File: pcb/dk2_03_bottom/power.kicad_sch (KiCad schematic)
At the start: 11 parts, among them J3 Eurorack_Power, U2 AP7333-33SAG, U8 XL1509-5.0

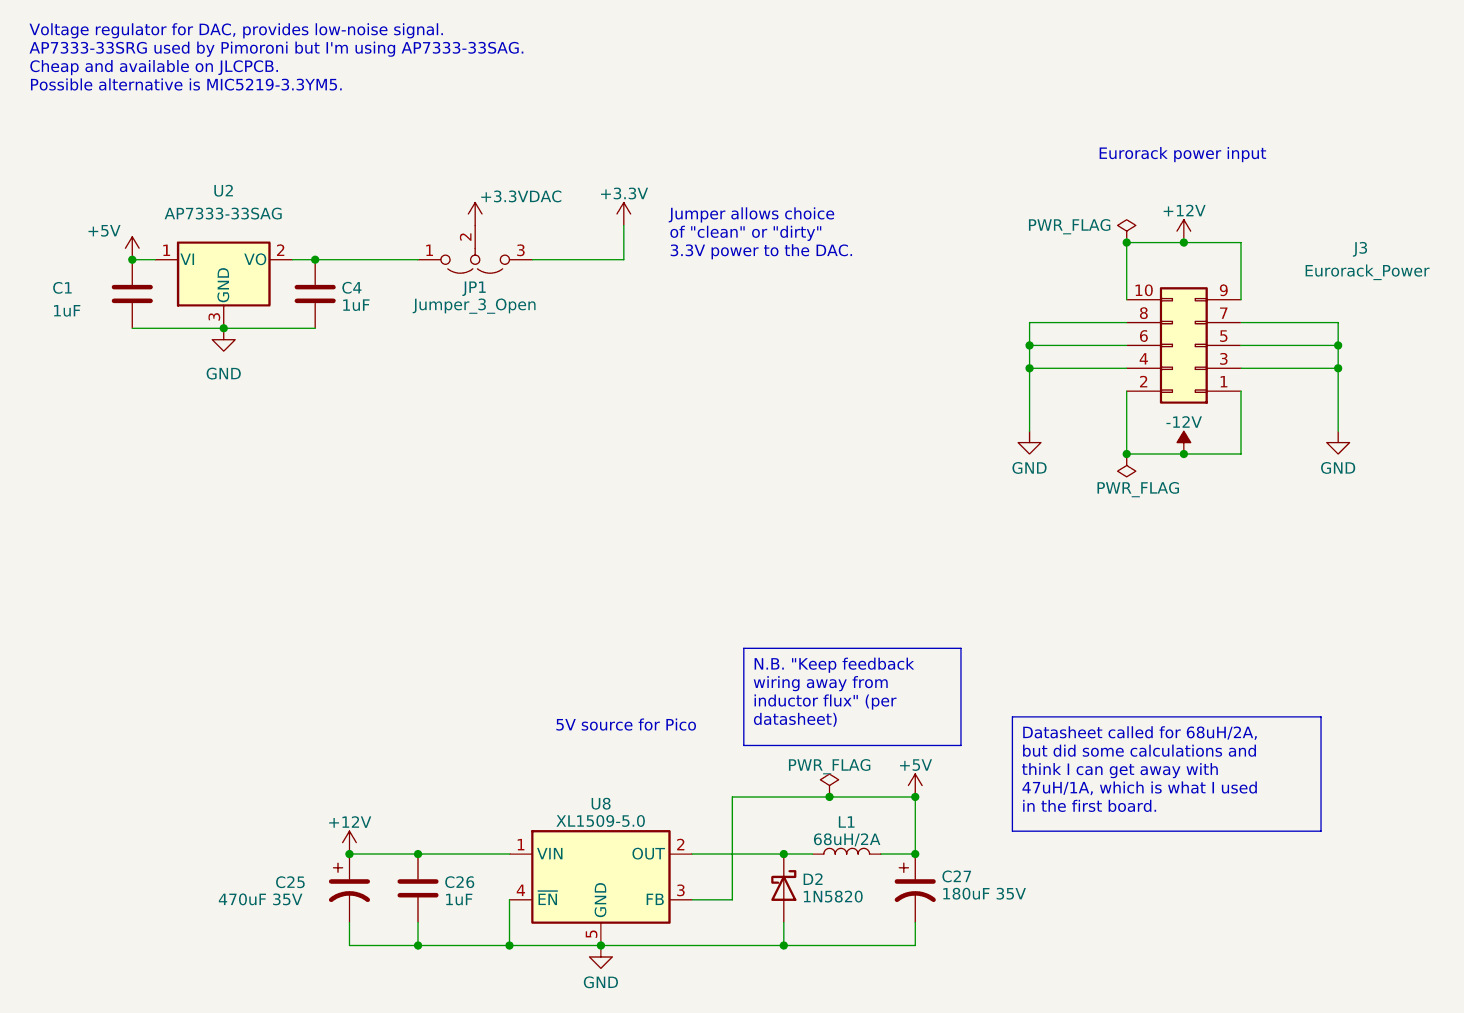
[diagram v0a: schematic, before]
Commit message: a commit before i mess up all the buttons
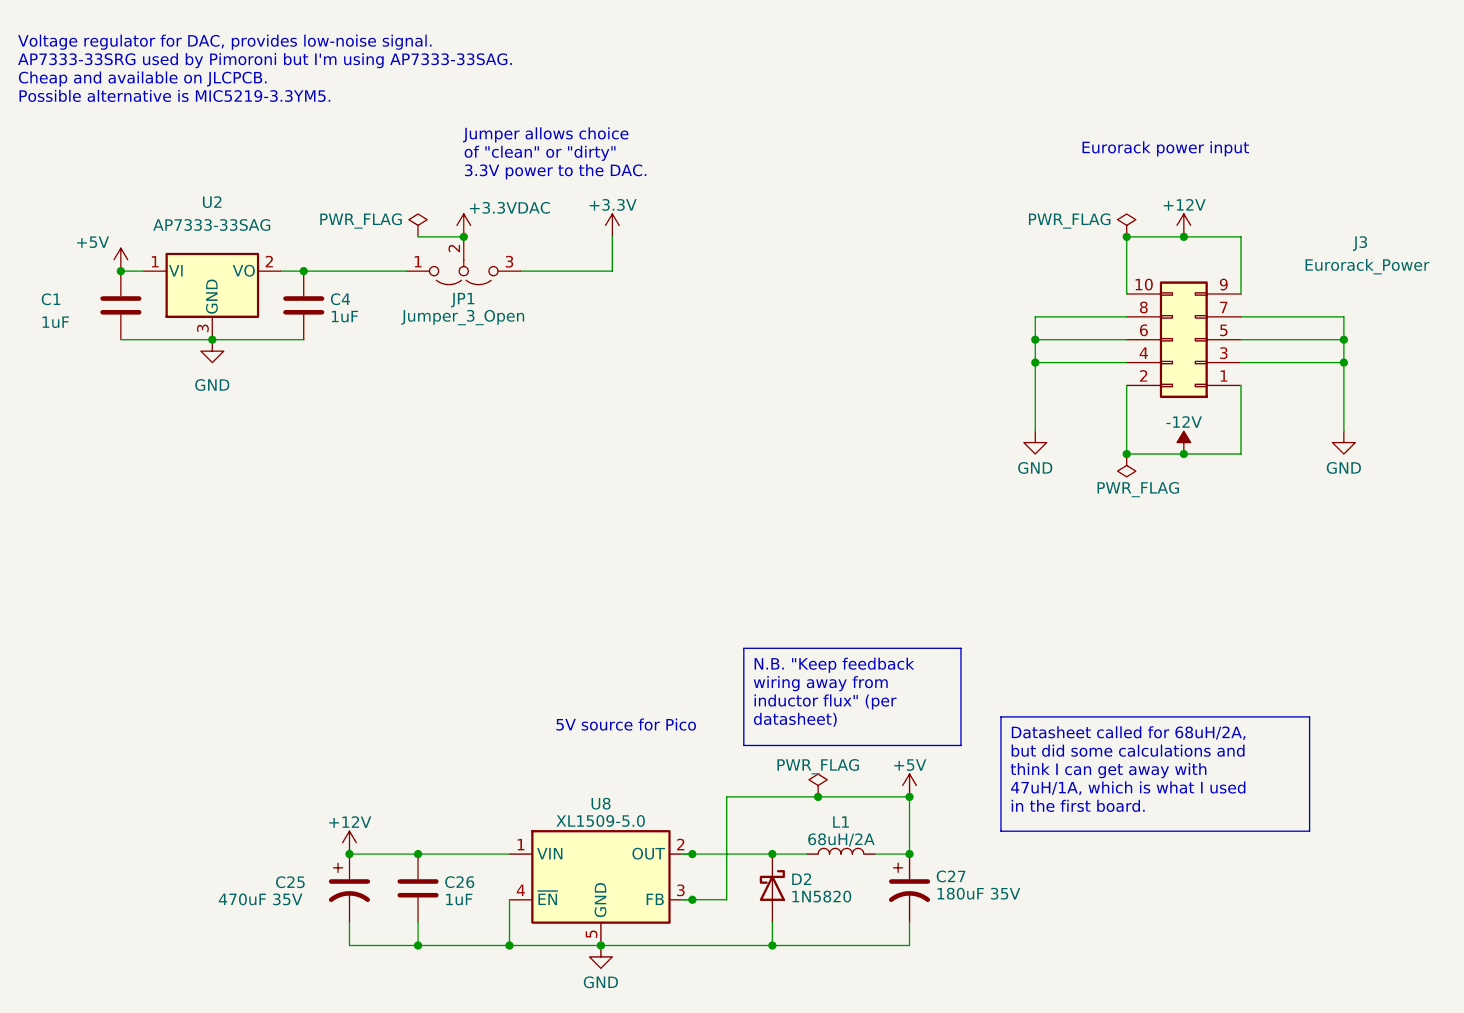
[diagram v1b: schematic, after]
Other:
- moved on the sheet: C1, C27, C4, D2, J3, JP1, L1, U2
